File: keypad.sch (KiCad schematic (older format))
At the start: 16 parts

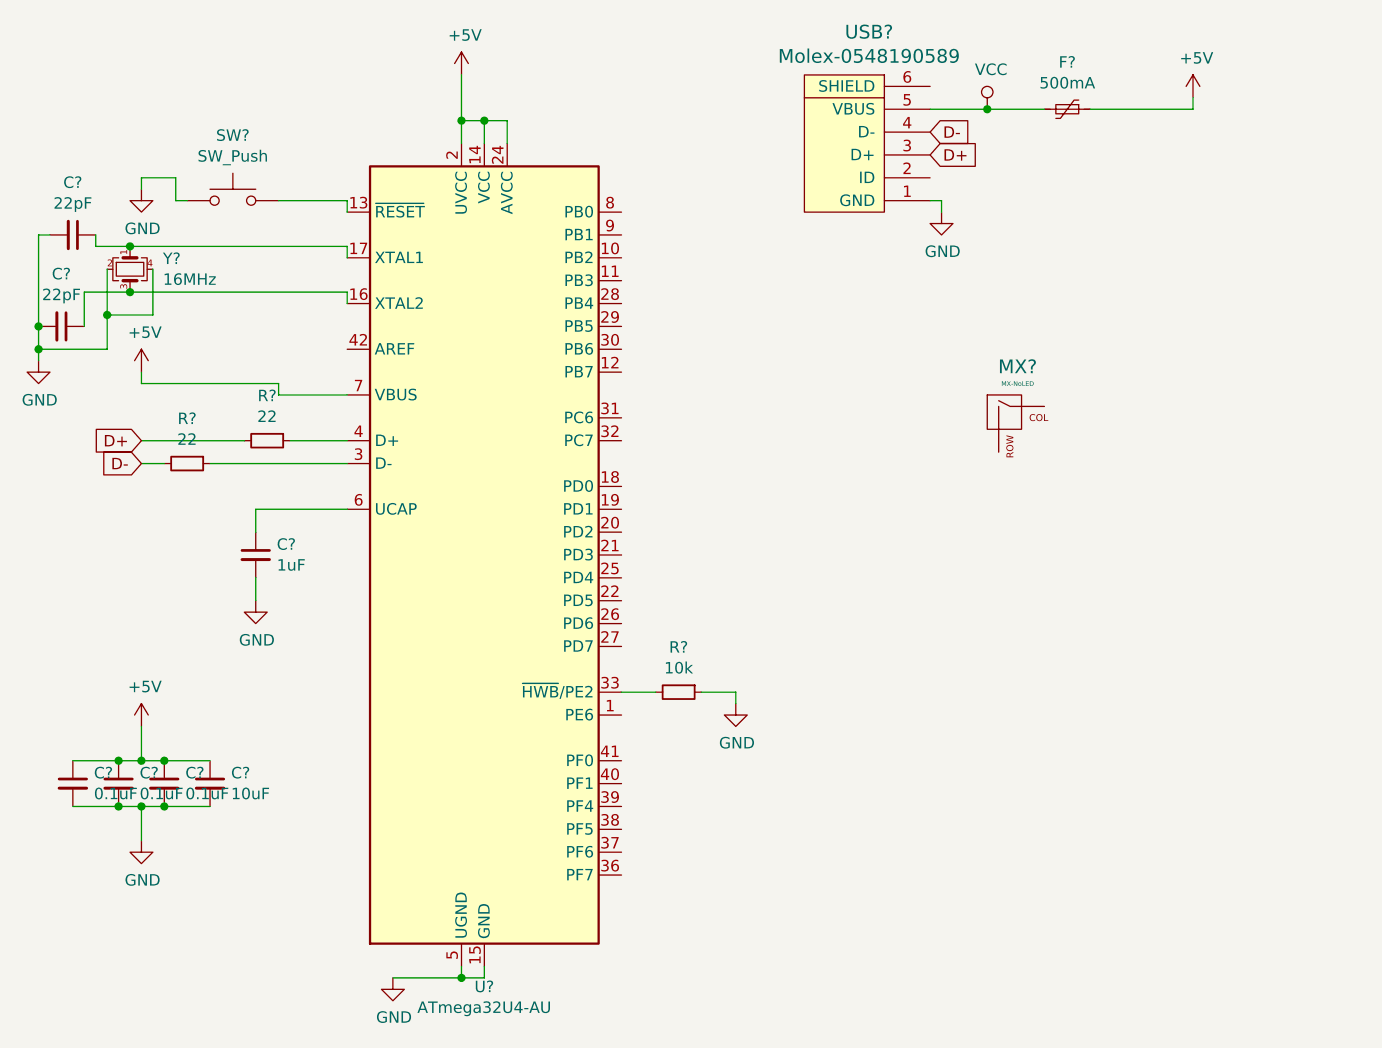
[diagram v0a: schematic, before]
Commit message: finished schematic
done
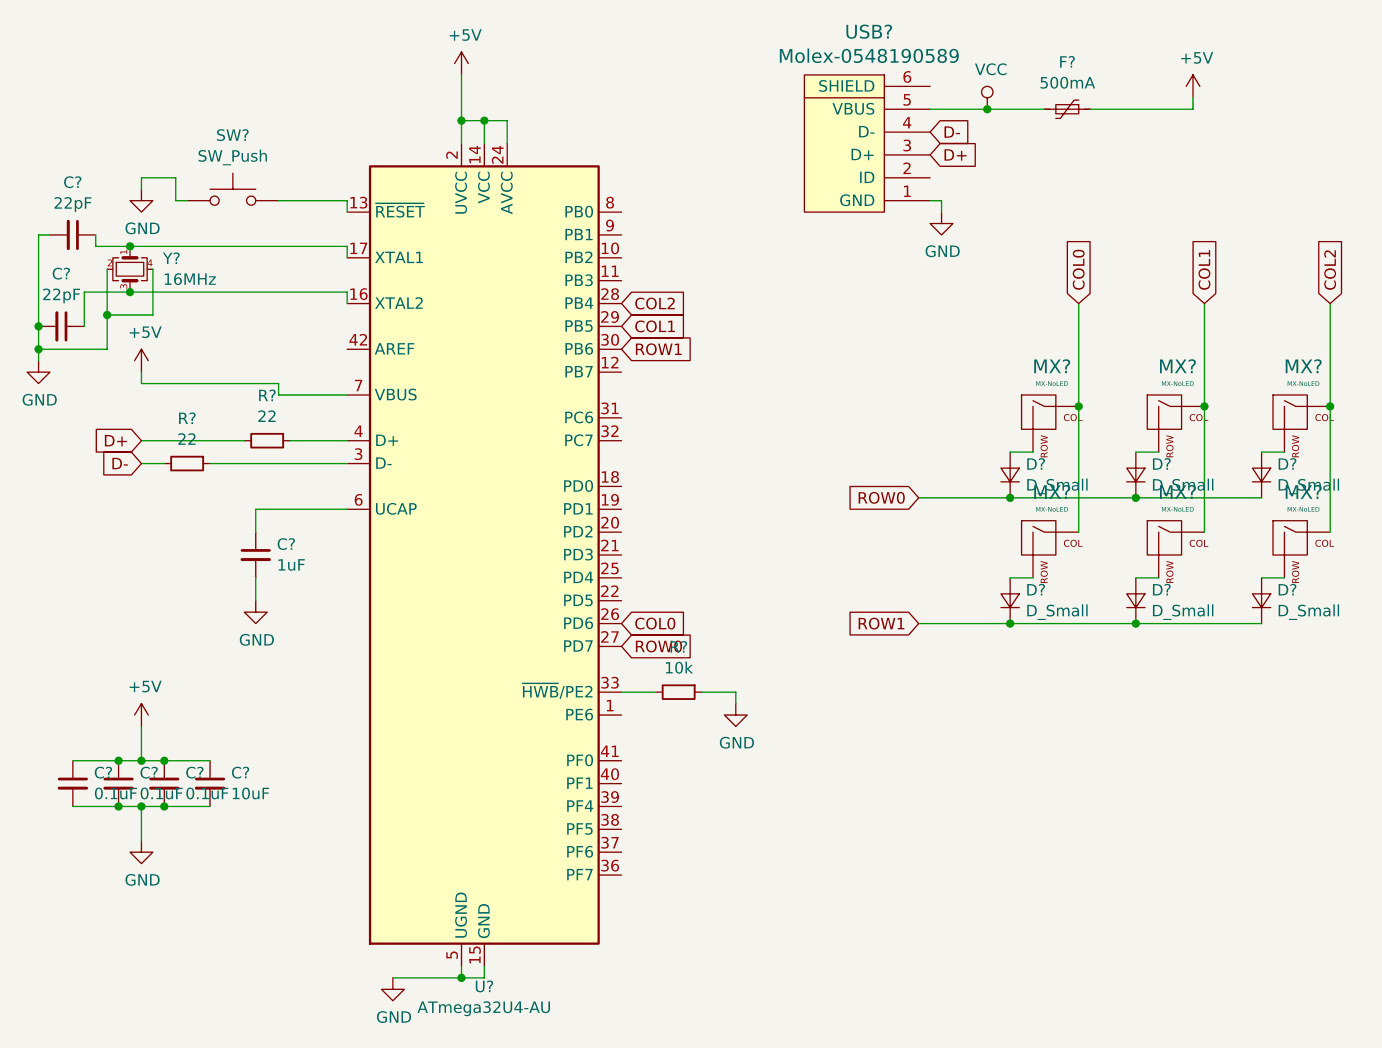
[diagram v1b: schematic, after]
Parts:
- added D? (x6): D_Small, symbol Device:D_Small
- added MX? (x5): MX-NoLED, symbol MX_Alps_Hybrid:MX-NoLED
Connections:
- net COL0: now reaches U?.26 (PD6)
- net COL0: now also MX?.1 (COL), MX?.1 (COL)
- net ROW0: now reaches U?.27 (PD7)
- net ROW0: now also D?.1 (K), D?.1 (K), D?.1 (K)
- net COL2: now reaches U?.28 (PB4)
- net COL2: now also MX?.1 (COL), MX?.1 (COL)
- net COL1: now reaches U?.29 (PB5)
- net COL1: now also MX?.1 (COL), MX?.1 (COL)
- net ROW1: now reaches U?.30 (PB6)
- net ROW1: now also D?.1 (K), D?.1 (K), D?.1 (K)
- net at MX?.2 (ROW): now also D?.2 (A)
- new net: D?.2 (A), MX?.2 (ROW) (x5)
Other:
- moved on the sheet: MX?
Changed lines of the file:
@@
 L MX_Alps_Hybrid:MX-NoLED MX?
 U 1 1 64704DD4
-P 5700 3600
-F 0 "MX?" H 5733 3823 60  0000 C CNN
-F 1 "MX-NoLED" H 5733 3749 20  0000 C CNN
-F 2 "" H 5075 3575 60  0001 C CNN
-F 3 "" H 5075 3575 60  0001 C CNN
-	1    5700 3600
+P 5850 3600
+F 0 "MX?" H 5883 3823 60  0000 C CNN
+F 1 "MX-NoLED" H 5883 3749 20  0000 C CNN
+F 2 "" H 5225 3575 60  0001 C CNN
+F 3 "" H 5225 3575 60  0001 C CNN
+	1    5850 3600
 	1    0    0    -1
 $EndComp
+$Comp
+L MX_Alps_Hybrid:MX-NoLED MX?
+U 1 1 64708931
+P 5850 4150
+F 0 "MX?" H 5883 4373 60  0000 C CNN
+F 1 "MX-NoLED" H 5883 4299 20  0000 C CNN
+F 2 "" H 5225 4125 60  0001 C CNN
+F 3 "" H 5225 4125 60  0001 C CNN
+	1    5850 4150
+	1    0    0    -1
+$EndComp
+$Comp
+L MX_Alps_Hybrid:MX-NoLED MX?
+U 1 1 64709440
+P 6400 3600
+F 0 "MX?" H 6433 3823 60  0000 C CNN
+F 1 "MX-NoLED" H 6433 3749 20  0000 C CNN
+F 2 "" H 5775 3575 60  0001 C CNN
+F 3 "" H 5775 3575 60  0001 C CNN
+	1    6400 3600
+	1    0    0    -1
+$EndComp
+$Comp
+L MX_Alps_Hybrid:MX-NoLED MX?
+U 1 1 64709B8A
+P 6400 4150
+F 0 "MX?" H 6433 4373 60  0000 C CNN
+F 1 "MX-NoLED" H 6433 4299 20  0000 C CNN
+F 2 "" H 5775 4125 60  0001 C CNN
+F 3 "" H 5775 4125 60  0001 C CNN
+	1    6400 4150
+	1    0    0    -1
+$EndComp
+$Comp
+L MX_Alps_Hybrid:MX-NoLED MX?
+U 1 1 6470A559
+P 6950 3600
+F 0 "MX?" H 6983 3823 60  0000 C CNN
+F 1 "MX-NoLED" H 6983 3749 20  0000 C CNN
+F 2 "" H 6325 3575 60  0001 C CNN
+F 3 "" H 6325 3575 60  0001 C CNN
+	1    6950 3600
+	1    0    0    -1
+$EndComp
+$Comp
+L MX_Alps_Hybrid:MX-NoLED MX?
+U 1 1 6470AC44
+P 6950 4150
+F 0 "MX?" H 6983 4373 60  0000 C CNN
+F 1 "MX-NoLED" H 6983 4299 20  0000 C CNN
+F 2 "" H 6325 4125 60  0001 C CNN
+F 3 "" H 6325 4125 60  0001 C CNN
+	1    6950 4150
+	1    0    0    -1
+$EndComp
+$Comp
+L Device:D_Small D?
+U 1 1 6470E23D
+P 5700 3850
+F 0 "D?" V 5746 3782 50  0000 R CNN
+F 1 "D_Small" V 5655 3782 50  0000 R CNN
+F 2 "" V 5700 3850 50  0001 C CNN
+F 3 "~" V 5700 3850 50  0001 C CNN
+	1    5700 3850
+	0    -1   -1   0
+$EndComp
+$Comp
+L Device:D_Small D?
+U 1 1 6470FC65
+P 6250 3850
+F 0 "D?" V 6296 3782 50  0000 R CNN
+F 1 "D_Small" V 6205 3782 50  0000 R CNN
+F 2 "" V 6250 3850 50  0001 C CNN
+F 3 "~" V 6250 3850 50  0001 C CNN
+	1    6250 3850
+	0    -1   -1   0
+$EndComp
+$Comp
+L Device:D_Small D?
+U 1 1 64710044
+P 6800 3850
+F 0 "D?" V 6846 3782 50  0000 R CNN
+F 1 "D_Small" V 6755 3782 50  0000 R CNN
+F 2 "" V 6800 3850 50  0001 C CNN
+F 3 "~" V 6800 3850 50  0001 C CNN
+	1    6800 3850
+	0    -1   -1   0
+$EndComp
+$Comp
+L Device:D_Small D?
+U 1 1 64710419
+P 6800 4400
+F 0 "D?" V 6846 4332 50  0000 R CNN
+F 1 "D_Small" V 6755 4332 50  0000 R CNN
+F 2 "" V 6800 4400 50  0001 C CNN
+F 3 "~" V 6800 4400 50  0001 C CNN
+	1    6800 4400
+	0    -1   -1   0
+$EndComp
+$Comp
+L Device:D_Small D?
+U 1 1 64710CE9
+P 6250 4400
+F 0 "D?" V 6296 4332 50  0000 R CNN
+F 1 "D_Small" V 6205 4332 50  0000 R CNN
+F 2 "" V 6250 4400 50  0001 C CNN
+F 3 "~" V 6250 4400 50  0001 C CNN
+	1    6250 4400
+	0    -1   -1   0
+$EndComp
+$Comp
+L Device:D_Small D?
+U 1 1 6471111D
+P 5700 4400
+F 0 "D?" V 5746 4332 50  0000 R CNN
+F 1 "D_Small" V 5655 4332 50  0000 R CNN
+F 2 "" V 5700 4400 50  0001 C CNN
+F 3 "~" V 5700 4400 50  0001 C CNN
+	1    5700 4400
+	0    -1   -1   0
+$EndComp
+Wire Wire Line
+	6000 4100 6000 3550
+Connection ~ 6000 3550
+Wire Wire Line
+	6000 3550 6000 3100
+Wire Wire Line
+	6550 4100 6550 3550
+Connection ~ 6550 3550
+Wire Wire Line
+	6550 3550 6550 3100
+Wire Wire Line
+	7100 4100 7100 3550
+Connection ~ 7100 3550
+Wire Wire Line
+	7100 3550 7100 3100
+Wire Wire Line
+	6900 3750 6800 3750
+Wire Wire Line
+	6900 4300 6800 4300
+Wire Wire Line
+	6350 4300 6250 4300
+Wire Wire Line
+	6350 3750 6250 3750
+Wire Wire Line
+	5800 3750 5700 3750
+Wire Wire Line
+	5800 4300 5700 4300
+Wire Wire Line
+	6800 3950 6250 3950
+Connection ~ 5700 3950
+Wire Wire Line
+	5700 3950 5300 3950
+Connection ~ 6250 3950
+Wire Wire Line
+	6250 3950 5700 3950
+Wire Wire Line
+	6800 4500 6250 4500
+Connection ~ 5700 4500
+Wire Wire Line
+	5700 4500 5300 4500
+Connection ~ 6250 4500
+Wire Wire Line
+	6250 4500 5700 4500
+Text GLabel 6000 3100 1    50   Input ~ 0
+COL0
+Text GLabel 6550 3100 1    50   Input ~ 0
+COL1
+Text GLabel 7100 3100 1    50   Input ~ 0
+COL2
+Text GLabel 5300 3950 0    50   Input ~ 0
+ROW0
+Text GLabel 5300 4500 0    50   Input ~ 0
+ROW1
+Text GLabel 4000 3300 2    50   Input ~ 0
+ROW1
+Text GLabel 4000 3100 2    50   Input ~ 0
+COL2
+Text GLabel 4000 3200 2    50   Input ~ 0
+COL1
+Text GLabel 4000 4600 2    50   Input ~ 0
+ROW0
+Text GLabel 4000 4500 2    50   Input ~ 0
+COL0
 $EndSCHEMATC
